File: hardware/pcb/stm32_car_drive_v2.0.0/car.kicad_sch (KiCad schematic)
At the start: 41 parts, among them J0 OLED, J14 OLED, J15 Conn_01x02, J17 Conn_01x05, J18 Conn_01x02, J19 Conn_01x02, J20 Conn_01x09, J22 Conn_01x10, J24 Conn_01x02, J25 HC-05, J26 Conn_01x08, J3 HC-05, K210 Conn_01x04, P1 USB_C_Plug_USB2.0, Q1 S8050, SW1 K1, SW2 K2, SW3 K3, SW4 K6, SW5 K5, SW6 K4, U10 CH340C

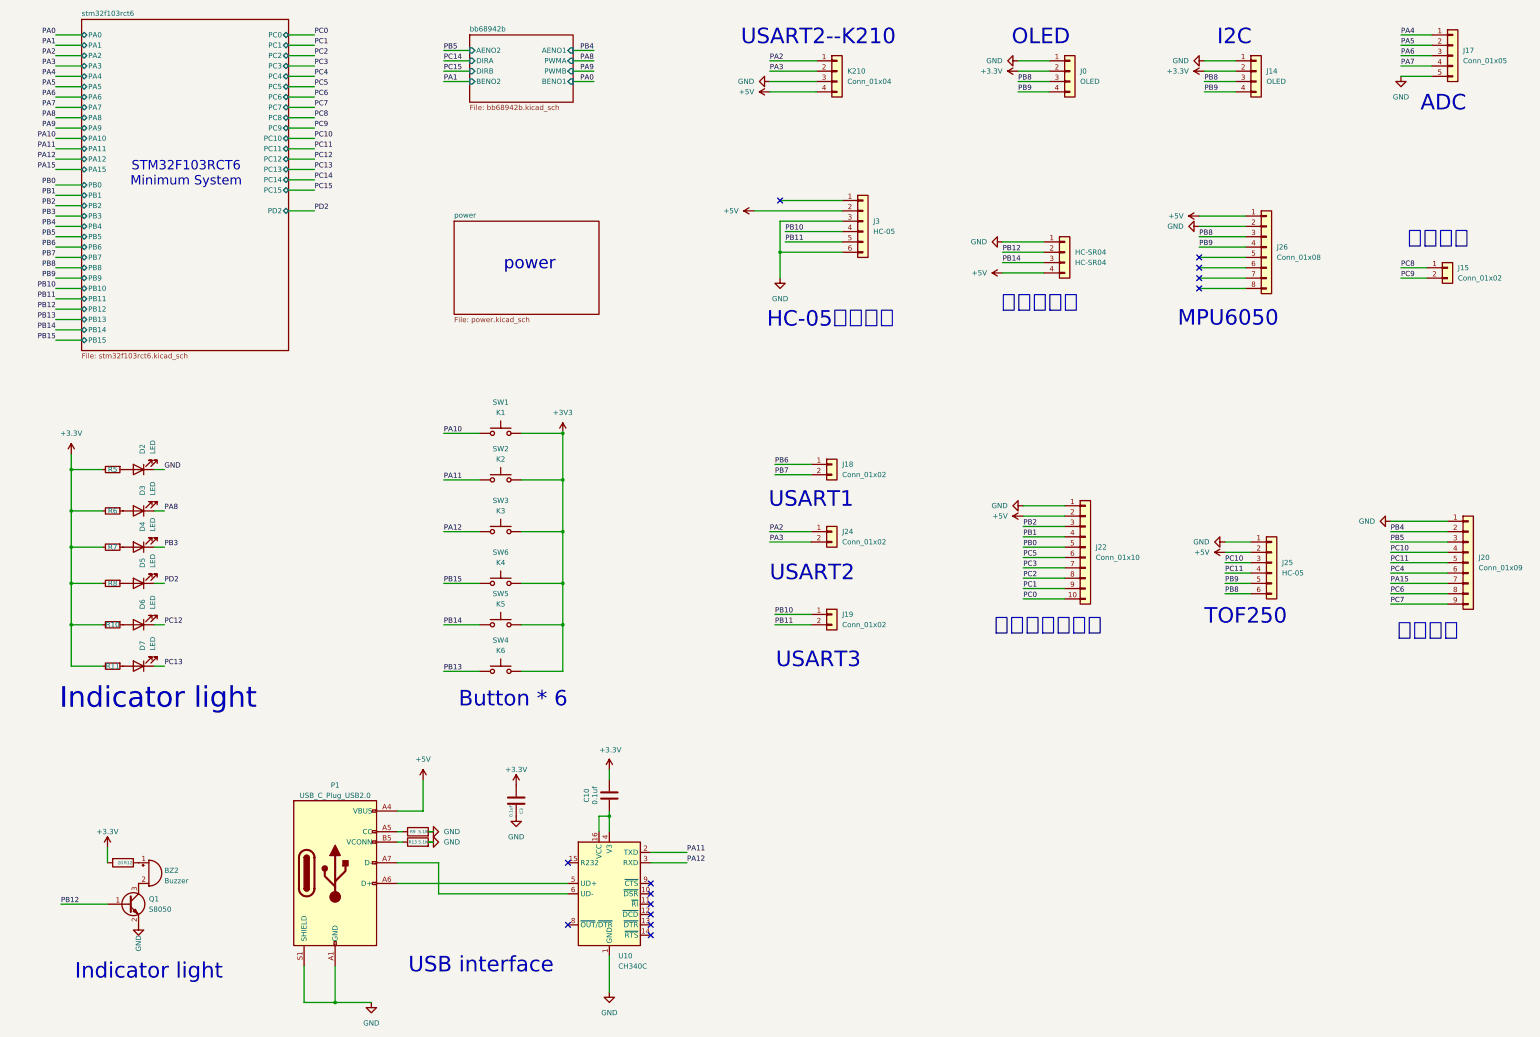
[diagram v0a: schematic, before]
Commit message: update
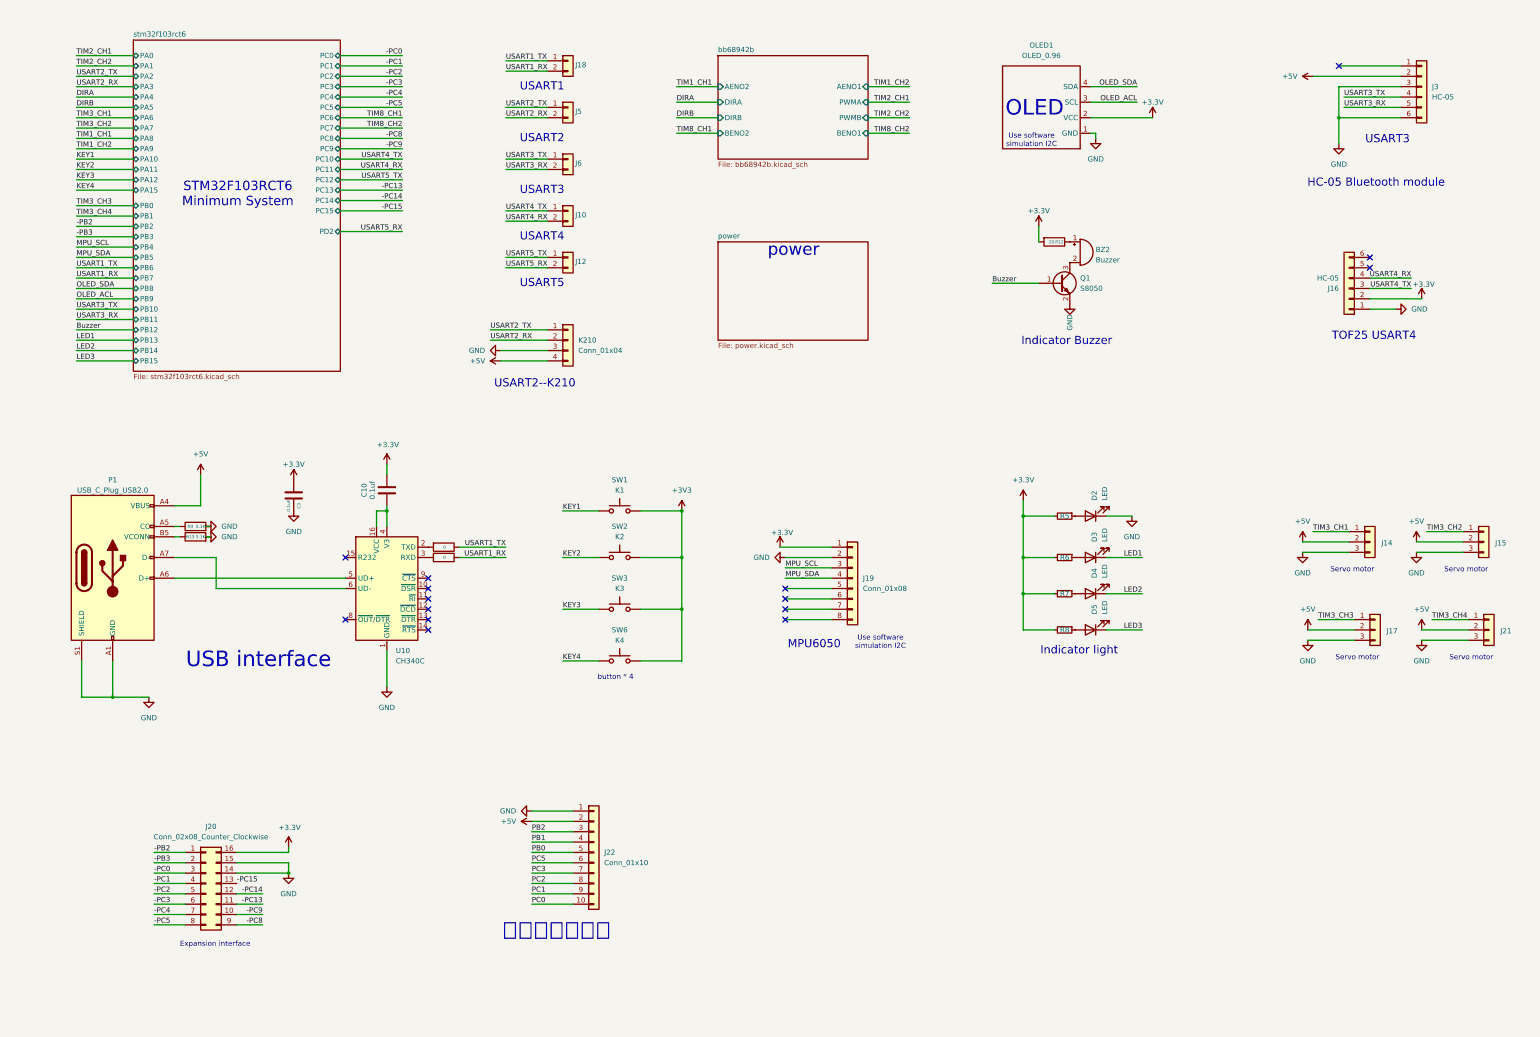
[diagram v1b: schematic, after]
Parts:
- removed D6, D7: LED, LED_SMD:LED_0805_2012Metric, symbol Library:LED
- removed HC-SR04: HC-SR04, Connector_PinSocket_2.54mm:PinSocket_1x04_P2.54mm_Vertical, symbol Library:Conn_01x04
- removed J0, J14: OLED, Connector_PinSocket_2.54mm:PinSocket_1x04_P2.54mm_Vertical, symbol Library:Conn_01x04
- removed J15: Conn_01x02, myself:HDR-TH_2P-P2.00-V-F-1, symbol Library:Conn_01x02
- removed J17: Conn_01x05, Connector_PinSocket_2.54mm:PinSocket_1x05_P2.54mm_Vertical, symbol Library:Conn_01x05
- removed J19, J24: Conn_01x02, Connector_PinSocket_2.54mm:PinSocket_1x02_P2.54mm_Vertical, symbol Library:Conn_01x02
- removed J20: Conn_01x09, Connector_PinSocket_2.54mm:PinSocket_1x09_P2.54mm_Vertical, symbol Library:Conn_01x09
- removed J25: HC-05, Connector_PinSocket_2.54mm:PinSocket_1x06_P2.54mm_Vertical, symbol Library:Conn_01x06
- removed J26: Conn_01x08, Connector_PinHeader_2.54mm:PinHeader_1x06_P2.54mm_Vertical, symbol Library:Conn_01x08
- removed R10, R11: 10k, Resistor_SMD:R_0603_1608Metric, symbol Library:R_Small
- removed SW4: K6, DuRuofu_Switch:SW_Push_1P1T_NO_6x6mm, symbol Library:SW_Push
- removed SW5: K5, DuRuofu_Switch:SW_Push_1P1T_NO_6x6mm, symbol Library:SW_Push
- added J10, J12, J5, J6: Conn_01x02, Connector_PinHeader_2.54mm:PinHeader_1x02_P2.54mm_Vertical, symbol Library:Conn_01x02
- added J14, J15, J17, J21: Conn_01x03, Connector_PinHeader_2.54mm:PinHeader_1x03_P2.54mm_Vertical, symbol Connector_Generic:Conn_01x03
- added J16: HC-05, Connector_PinSocket_2.54mm:PinSocket_1x06_P2.54mm_Vertical, symbol Library:Conn_01x06
- added J19: Conn_01x08, DuRuofu_Module:MPU6050-GY-521, symbol Library:Conn_01x08
- added J20: Conn_02x08_Counter_Clockwise, Connector_PinHeader_2.54mm:PinHeader_2x08_P2.54mm_Vertical, symbol Connector_Generic:Conn_02x08_Counter_Clockwise
- added OLED1: OLED_0.96, DuRuofu_Module:0.96OLED_4P, symbol DuRuofu_Module:0.96OLED_4P
- added R3, R4: 0, Resistor_SMD:R_0603_1608Metric, symbol Library:R
- J18: footprint Connector_PinSocket_2.54mm:PinSocket_1x02_P2.54mm_Vertical -> Connector_PinHeader_2.54mm:PinHeader_1x02_P2.54mm_Vertical
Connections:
- net +3.3V: now also J16.2 (Pin_2), J19.1 (Pin_1), J20.16 (Pin_16), OLED1.2 (VCC)
- net +5V: now also J14.2 (Pin_2), J15.2 (Pin_2), J17.2 (Pin_2), J21.2 (Pin_2)
- net GND: now also J14.3 (Pin_3), J15.3 (Pin_3), J16.1 (Pin_1), J17.3 (Pin_3), J19.2 (Pin_2), J20.14 (Pin_14), J20.15 (Pin_15), J21.3 (Pin_3), OLED1.1 (GND)
- net PA10 renamed KEY1
- net PA11: no longer names the net of U10.2 (TXD)
- net PA11: now also R3.2; no longer SW2.1
- net PA12: no longer names the net of U10.3 (RXD)
- net PA12: now also R4.2; no longer SW3.1
- net PA2 renamed USART2_TX
- net USART2_TX: now also J5.1 (Pin_1)
- net PA3 renamed USART2_RX
- net USART2_RX: now also J5.2 (Pin_2)
- net PA8 renamed LED1
- net PB10 renamed USART3_TX
- net USART3_TX: now also J6.1 (Pin_1)
- net PB11 renamed USART3_RX
- net USART3_RX: now also J6.2 (Pin_2)
- net PB12 renamed Buzzer
- net PB15 renamed KEY4
- net PB3 renamed LED2
- net PB6 renamed USART1_TX
- net USART1_TX: now also R3.1
- net PB7 renamed USART1_RX
- net USART1_RX: now also R4.1
- net PD2 renamed LED3
- new net -PB2: J20.1 (Pin_1)
- new net -PB3: J20.2 (Pin_2)
- new net -PC0: J20.3 (Pin_3)
- new net -PC1: J20.4 (Pin_4)
- new net -PC13: J20.11 (Pin_11)
- new net -PC14: J20.12 (Pin_12)
- new net -PC15: J20.13 (Pin_13)
- new net -PC2: J20.5 (Pin_5)
- new net -PC3: J20.6 (Pin_6)
- new net -PC4: J20.7 (Pin_7)
- new net -PC5: J20.8 (Pin_8)
- new net -PC8: J20.9 (Pin_9)
- new net -PC9: J20.10 (Pin_10)
- new net KEY2: SW2.1
- new net KEY3: SW3.1
- new net MPU_SCL: J19.3 (Pin_3)
- new net MPU_SDA: J19.4 (Pin_4)
- new net OLED_ACL: OLED1.3 (SCL)
- new net OLED_SDA: OLED1.4 (SDA)
- new net TIM3_CH1: J14.1 (Pin_1)
- new net TIM3_CH2: J15.1 (Pin_1)
- new net TIM3_CH3: J17.1 (Pin_1)
- new net TIM3_CH4: J21.1 (Pin_1)
- new net USART4_RX: J10.2 (Pin_2), J16.4 (Pin_4)
- new net USART4_TX: J10.1 (Pin_1), J16.3 (Pin_3)
- new net USART5_RX: J12.2 (Pin_2)
- new net USART5_TX: J12.1 (Pin_1)
- no-connect marks 13 -> 15
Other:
- note added: "Expansion interface"
- note added: "HC-05 Bluetooth module"
- note added: "Indicator Buzzer"
- note added: "Servo motor"
- note added: "TOF25 USART4"
- note added: "USART4"
- note added: "USART5"
- note added: "Use software simulation I2C"
- note added: "button * 4"
- note removed: "ADC"
- note removed: "Button * 6"
- note removed: "HC-05蓝牙模块"
- note removed: "I2C"
- note removed: "TOF250"
- note removed: "多余接口"
- note removed: "舵机驱动"
- note removed: "超声波测距"
- moved on the sheet: BZ2, C10, C3, D2, D3, D4, D5, J18, J22, J3, K210, P1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
